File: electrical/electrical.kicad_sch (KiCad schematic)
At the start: 0 parts

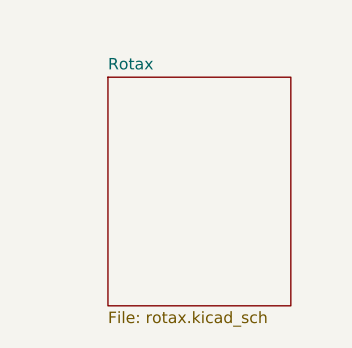
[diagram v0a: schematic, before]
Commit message: Added rotax
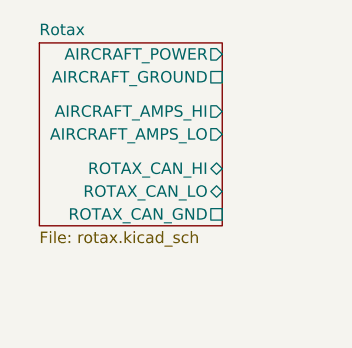
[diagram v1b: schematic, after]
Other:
- sheet Rotax ports: added AIRCRAFT_AMPS_HI, AIRCRAFT_AMPS_LO, AIRCRAFT_GROUND, AIRCRAFT_POWER, ROTAX_CAN_GND, ROTAX_CAN_HI, ROTAX_CAN_LO; removed none
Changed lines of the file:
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@@
     (company "N915SN Angry Bird")
   )
-  (sheet (at 26.67 22.86) (size 20.32 25.4) (fields_autoplaced)
+  (sheet (at 19.05 19.05) (size 20.32 20.32) (fields_autoplaced)
     (stroke (width 0.1524) (type solid))
     (fill (color 0 0 0 0.0000))
-    (property "Sheetname" "Rotax" (at 26.67 22.1484 0)
+    (property "Sheetname" "Rotax" (at 19.05 18.3384 0)
       (effects (font (size 1.27 1.27)) (justify left bottom))
     )
-    (property "Sheetfile" "rotax.kicad_sch" (at 26.67 48.8446 0)
+    (property "Sheetfile" "rotax.kicad_sch" (at 19.05 39.9546 0)
       (effects (font (size 1.27 1.27)) (justify left top))
     )
+    (pin "AIRCRAFT_POWER" output (at 39.37 20.32 0)
+      (effects (font (size 1.27 1.27)) (justify right))
+    )
+    (pin "AIRCRAFT_GROUND" passive (at 39.37 22.86 0)
+      (effects (font (size 1.27 1.27)) (justify right))
+    )
+    (pin "AIRCRAFT_AMPS_HI" output (at 39.37 26.67 0)
+      (effects (font (size 1.27 1.27)) (justify right))
+    )
+    (pin "AIRCRAFT_AMPS_LO" output (at 39.37 29.21 0)
+      (effects (font (size 1.27 1.27)) (justify right))
+    )
+    (pin "ROTAX_CAN_LO" bidirectional (at 39.37 35.56 0)
+      (effects (font (size 1.27 1.27)) (justify right))
+    )
+    (pin "ROTAX_CAN_GND" passive (at 39.37 38.1 0)
+      (effects (font (size 1.27 1.27)) (justify right))
+    )
+    (pin "ROTAX_CAN_HI" bidirectional (at 39.37 33.02 0)
+      (effects (font (size 1.27 1.27)) (justify right))
+    )
     (instances
